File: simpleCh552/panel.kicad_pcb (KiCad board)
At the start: 2 copper layers, 42 x 56 mm, 60 parts, among them J1 Conn_01x02_Pin, J2 left, J3 Conn_01x03_Pin, SW1 SW_SPST, U1 CH552G

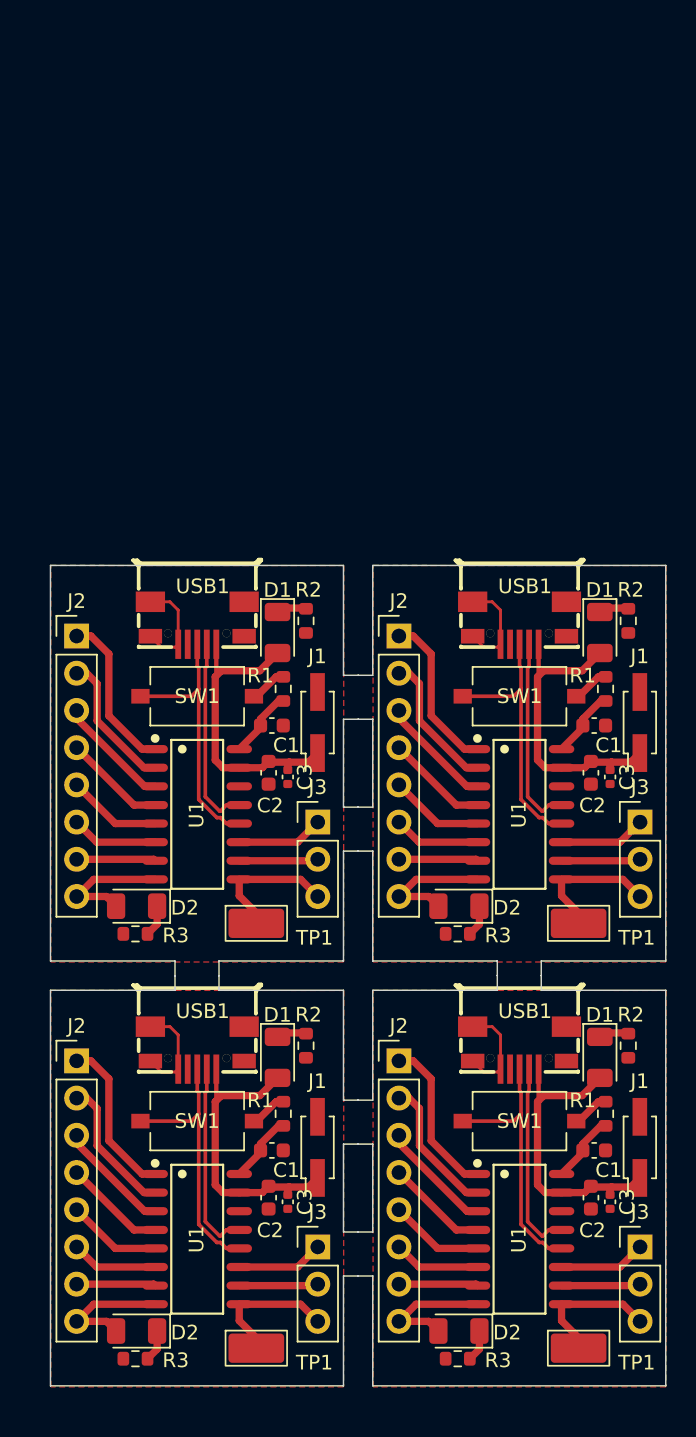
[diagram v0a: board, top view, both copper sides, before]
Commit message: update
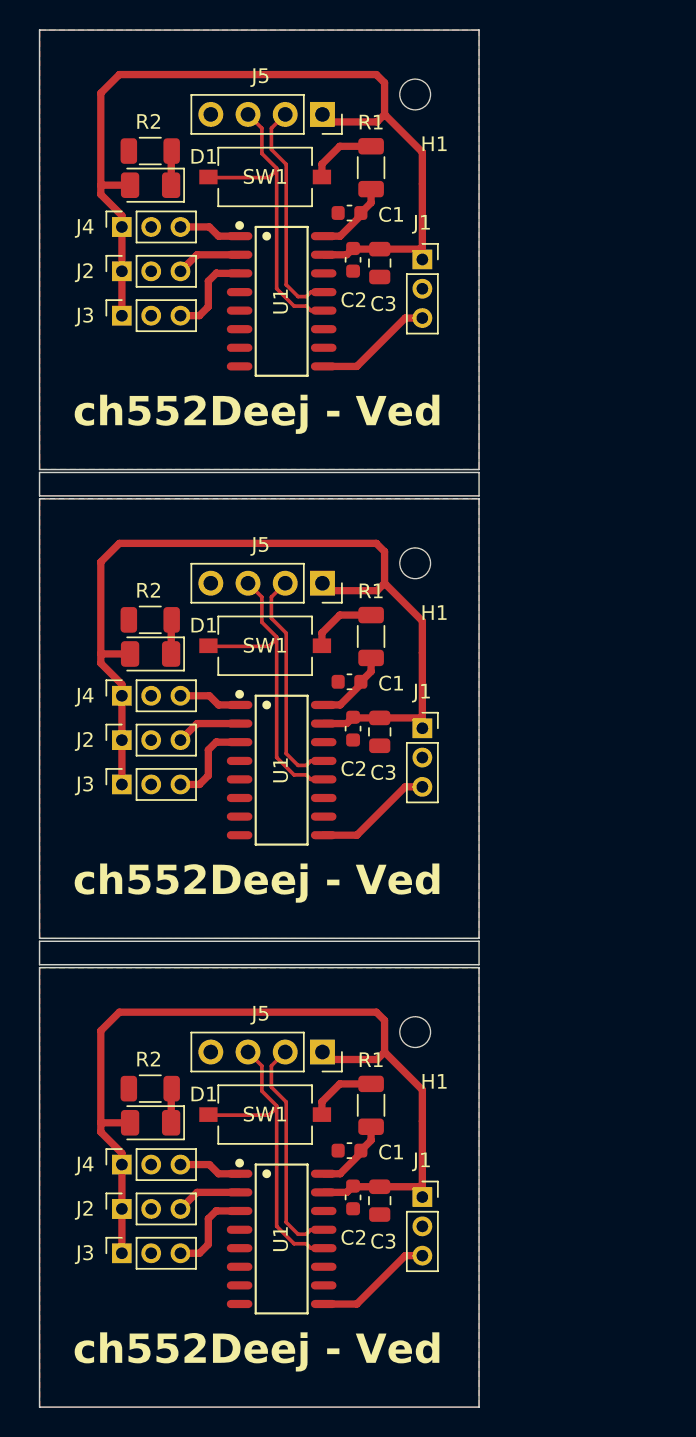
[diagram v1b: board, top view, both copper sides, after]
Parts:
- removed the C1 at (149.4, 96.5)
- removed the C1 at (149.4, 67.5)
- removed the C1 at (171.4, 96.5)
- removed the C1 at (171.4, 67.5)
- removed the C2 at (149.1, 99.7)
- removed the C2 at (149.1, 70.7)
- removed the C2 at (171.1, 99.7)
- removed the C2 at (171.1, 70.7)
- removed the C3 at (172.4, 71.0)
- removed the C3 at (172.4, 100.0)
- removed the C3 at (150.4, 71.0)
- removed the C3 at (150.4, 100.0)
- removed the D1 at (149.7, 61.1)
- removed the D1 at (171.7, 61.1)
- removed the D1 at (171.7, 90.1)
- removed the D1 at (149.7, 90.1)
- removed D2 (x4): LED, LED_SMD:LED_1206_3216Metric
- removed the J1 at (152.5, 96.3)
- removed the J1 at (152.5, 67.3)
- removed the J1 at (174.5, 67.3)
- removed the J1 at (174.5, 96.3)
- removed the J2 at (136.0, 90.4)
- removed the J2 at (136.0, 61.4)
- removed the J2 at (158.0, 61.4)
- removed the J2 at (158.0, 90.4)
- removed the J3 at (152.5, 74.1)
- removed the J3 at (174.5, 74.1)
- removed the J3 at (174.5, 103.1)
- removed the J3 at (152.5, 103.1)
- removed the R1 at (150.1, 94.0)
- removed the R1 at (172.1, 94.0)
- removed the R1 at (150.1, 65.0)
- removed the R1 at (172.1, 65.0)
- removed the R2 at (173.7, 60.3)
- removed the R2 at (173.7, 89.3)
- removed the R2 at (151.7, 60.3)
- removed the R2 at (151.7, 89.3)
- removed R3 (x4): 1k, Resistor_SMD:R_0603_1608Metric
- removed the SW1 at (144.3, 94.5)
- removed the SW1 at (166.3, 94.5)
- removed the SW1 at (166.3, 65.5)
- removed the SW1 at (144.3, 65.5)
- removed TP1 (x4): TestPoint, TestPoint:TestPoint_Keystone_5019_Miniature
- removed the U1 at (144.3, 102.5)
- removed the U1 at (166.3, 73.5)
- removed the U1 at (166.3, 102.5)
- removed the U1 at (144.3, 73.5)
- removed USB1 (x4): MICROQTJ, mylib:MICRO-USB-SMD_MICROQTJ-5P
- added C1: 100n, Capacitor_SMD:C_0603_1608Metric, F.Cu at (154.7, 32.5)
- added C1: 100n, Capacitor_SMD:C_0603_1608Metric, F.Cu at (154.7, 64.5)
- added C1: 100n, Capacitor_SMD:C_0603_1608Metric, F.Cu at (154.7, 96.5)
- added C2: 100n, Capacitor_SMD:C_0603_1608Metric, F.Cu at (154.9, 99.7)
- added C2: 100n, Capacitor_SMD:C_0603_1608Metric, F.Cu at (154.9, 35.7)
- added C2: 100n, Capacitor_SMD:C_0603_1608Metric, F.Cu at (154.9, 67.7)
- added C3: 10uf, Capacitor_SMD:C_0805_2012Metric, F.Cu at (156.7, 35.9)
- added C3: 10uf, Capacitor_SMD:C_0805_2012Metric, F.Cu at (156.7, 99.9)
- added C3: 10uf, Capacitor_SMD:C_0805_2012Metric, F.Cu at (156.7, 67.9)
- added D1: LED, LED_SMD:LED_1206_3216Metric, F.Cu at (141.1, 62.6)
- added D1: LED, LED_SMD:LED_1206_3216Metric, F.Cu at (141.1, 30.6)
- added D1: LED, LED_SMD:LED_1206_3216Metric, F.Cu at (141.1, 94.6)
- added H1: MountingHole, MountingHole:MountingHole_2.1mm, F.Cu at (159.1, 24.4)
- added H1: MountingHole, MountingHole:MountingHole_2.1mm, F.Cu at (159.1, 88.4)
- added H1: MountingHole, MountingHole:MountingHole_2.1mm, F.Cu at (159.1, 56.4)
- added J1: A0, Connector_PinSocket_2.00mm:PinSocket_1x03_P2.00mm_Vertical, F.Cu at (159.6, 67.7)
- added J1: A0, Connector_PinSocket_2.00mm:PinSocket_1x03_P2.00mm_Vertical, F.Cu at (159.6, 35.7)
- added J1: A0, Connector_PinSocket_2.00mm:PinSocket_1x03_P2.00mm_Vertical, F.Cu at (159.6, 99.7)
- added J2: A1, Connector_PinSocket_2.00mm:PinSocket_1x03_P2.00mm_Vertical, F.Cu at (139.1, 100.5)
- added J2: A1, Connector_PinSocket_2.00mm:PinSocket_1x03_P2.00mm_Vertical, F.Cu at (139.1, 68.5)
- added J2: A1, Connector_PinSocket_2.00mm:PinSocket_1x03_P2.00mm_Vertical, F.Cu at (139.1, 36.5)
- added J3: A2, Connector_PinSocket_2.00mm:PinSocket_1x03_P2.00mm_Vertical, F.Cu at (139.1, 71.5)
- added J3: A2, Connector_PinSocket_2.00mm:PinSocket_1x03_P2.00mm_Vertical, F.Cu at (139.1, 103.5)
- added J3: A2, Connector_PinSocket_2.00mm:PinSocket_1x03_P2.00mm_Vertical, F.Cu at (139.1, 39.5)
- added J4: A3, Connector_PinSocket_2.00mm:PinSocket_1x03_P2.00mm_Vertical, F.Cu at (139.1, 65.4)
- added J4: A3, Connector_PinSocket_2.00mm:PinSocket_1x03_P2.00mm_Vertical, F.Cu at (139.1, 33.4)
- added J4: A3, Connector_PinSocket_2.00mm:PinSocket_1x03_P2.00mm_Vertical, F.Cu at (139.1, 97.4)
- added J5: Conn_01x04, Connector_PinSocket_2.54mm:PinSocket_1x04_P2.54mm_Vertical, F.Cu at (152.8, 57.8)
- added J5: Conn_01x04, Connector_PinSocket_2.54mm:PinSocket_1x04_P2.54mm_Vertical, F.Cu at (152.8, 25.8)
- added J5: Conn_01x04, Connector_PinSocket_2.54mm:PinSocket_1x04_P2.54mm_Vertical, F.Cu at (152.8, 89.8)
- added R1: 10k, Resistor_SMD:R_1206_3216Metric, F.Cu at (156.1, 93.4)
- added R1: 10k, Resistor_SMD:R_1206_3216Metric, F.Cu at (156.1, 61.4)
- added R1: 10k, Resistor_SMD:R_1206_3216Metric, F.Cu at (156.1, 29.4)
- added R2: 1k, Resistor_SMD:R_1206_3216Metric, F.Cu at (141.1, 92.3)
- added R2: 1k, Resistor_SMD:R_1206_3216Metric, F.Cu at (141.1, 28.3)
- added R2: 1k, Resistor_SMD:R_1206_3216Metric, F.Cu at (141.1, 60.3)
- added SW1: SW_SPST, Button_Switch_SMD:SW_Tactile_SPST_NO_Straight_CK_PTS636Sx25SMTRLFS, F.Cu at (148.9, 30.0)
- added SW1: SW_SPST, Button_Switch_SMD:SW_Tactile_SPST_NO_Straight_CK_PTS636Sx25SMTRLFS, F.Cu at (148.9, 94.0)
- added SW1: SW_SPST, Button_Switch_SMD:SW_Tactile_SPST_NO_Straight_CK_PTS636Sx25SMTRLFS, F.Cu at (148.9, 62.0)
- added U1: CH552G, mylib:SOP-16_L10.0-W3.9-P1.27-LS6.0-BL, F.Cu at (150.0, 70.5)
- added U1: CH552G, mylib:SOP-16_L10.0-W3.9-P1.27-LS6.0-BL, F.Cu at (150.0, 102.5)
- added U1: CH552G, mylib:SOP-16_L10.0-W3.9-P1.27-LS6.0-BL, F.Cu at (150.0, 38.5)
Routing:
- net Board_1-VCC: track 21.1 -> 62.7 mm
- net Board_2-VCC: track 21.1 -> 62.7 mm
- net Board_0-VCC: track 21.1 -> 62.7 mm
- net Board_3-VCC: track 21.1 -> 0.00 mm
- net Board_3-/D+: track 18.3 -> 0.00 mm
- net Board_3-/D-: track 13.3 -> 0.00 mm
- net Board_3-Net-(J2-Pin_1): track 11.0 -> 0.00 mm
- net Board_2-Net-(J2-Pin_1): track 11.0 -> 0.00 mm
- net Board_1-Net-(J2-Pin_1): track 11.0 -> 0.00 mm
- net Board_0-Net-(J2-Pin_1): track 11.0 -> 0.00 mm
- net Board_3-Net-(J2-Pin_2): track 9.51 -> 0.00 mm
- net Board_2-Net-(J2-Pin_2): track 9.51 -> 0.00 mm
- net Board_1-Net-(J2-Pin_2): track 9.51 -> 0.00 mm
- net Board_0-Net-(J2-Pin_2): track 9.51 -> 0.00 mm
- net Board_3-/1.1: track 9.33 -> 0.00 mm
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- removed copper zone on F.Cu, net Board_3-GND
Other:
- board size 42 x 56 mm -> 30 x 94 mm
- board text added: "ch552Deej - Ved"
